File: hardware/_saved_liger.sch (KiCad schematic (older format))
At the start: 77 parts, among them P1 CONN_01X10, P2 CONN_01X10, P4 CONN_01X02, P5 CONN_01X04, Q1 Q_NMOS_GSD, Q2 Q_PMOS_GSD, Q3 Q_NPN_BEC, Q4 Q_NPN_BEC, SW1 SW_PUSH, U11 SPX3819, U2 ADA4075, U3 ESP-WROOM-02, U5 PT5529B/L2/H2-F

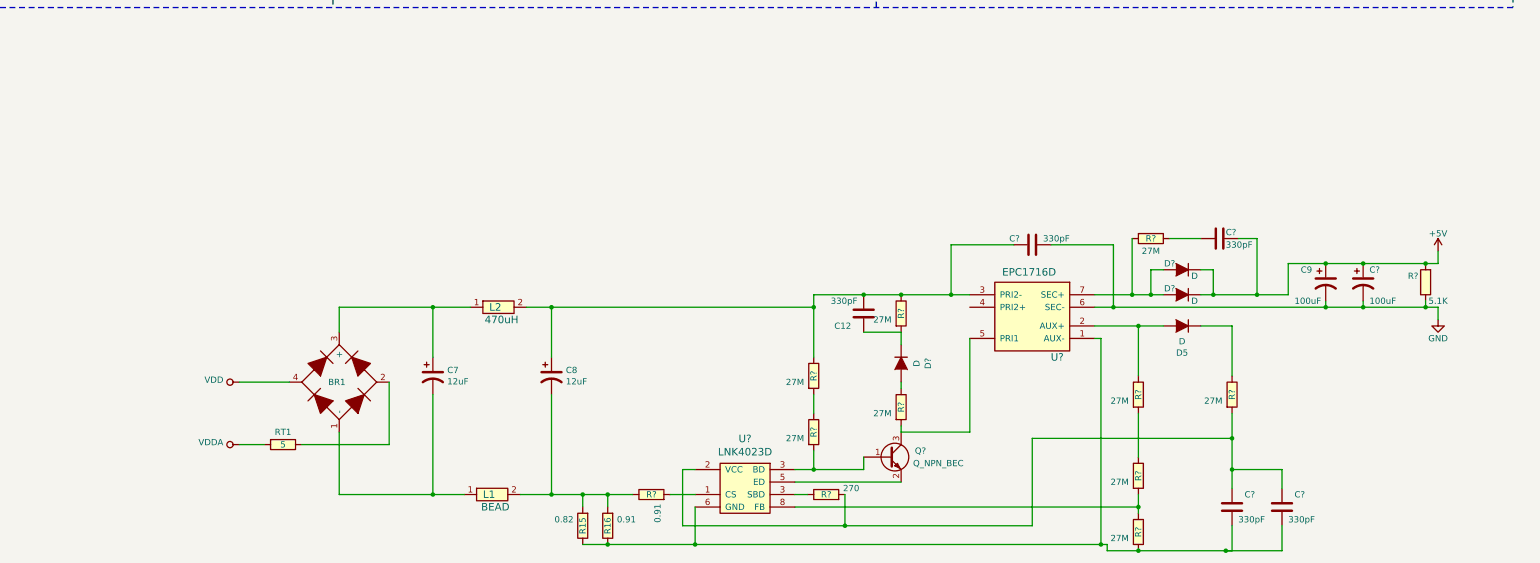
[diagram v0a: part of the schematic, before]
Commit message: update
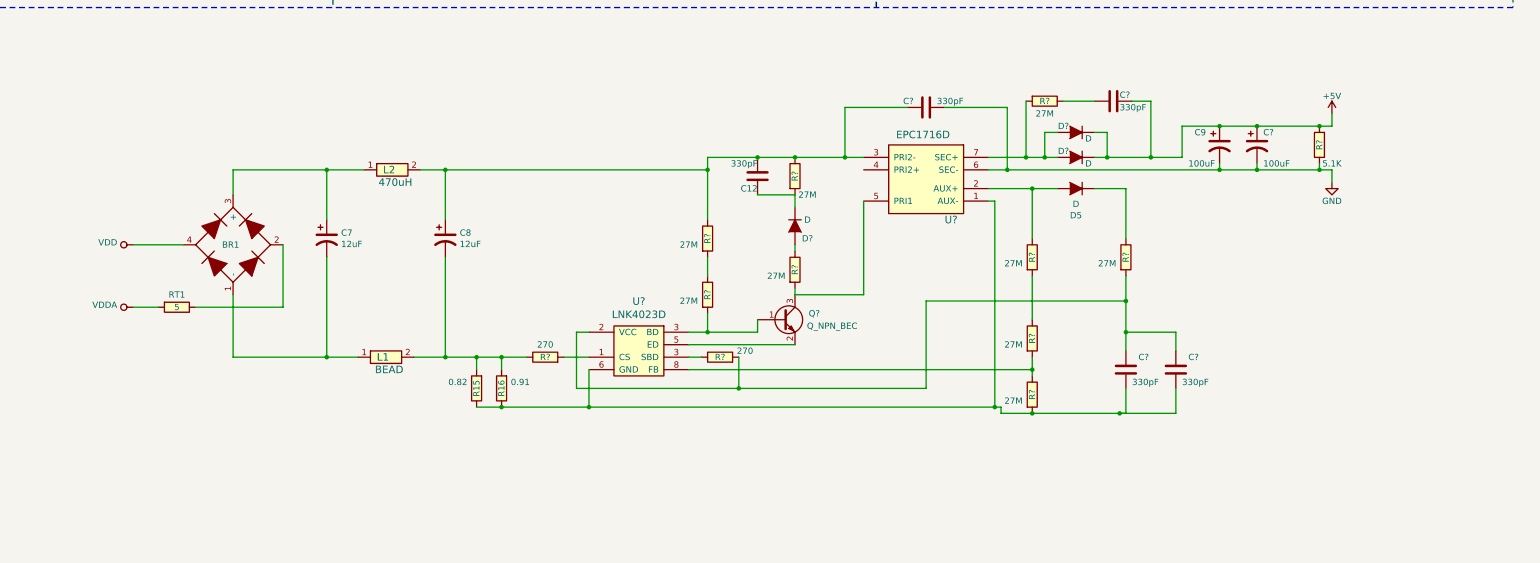
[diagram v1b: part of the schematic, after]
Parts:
- R?: value 0.91 -> 270
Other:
- moved on the sheet: BR1, C12, C7, C8, C9, C?, D5, D?, L1, L2, Q?, R15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
